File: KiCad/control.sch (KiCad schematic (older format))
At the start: 69 parts

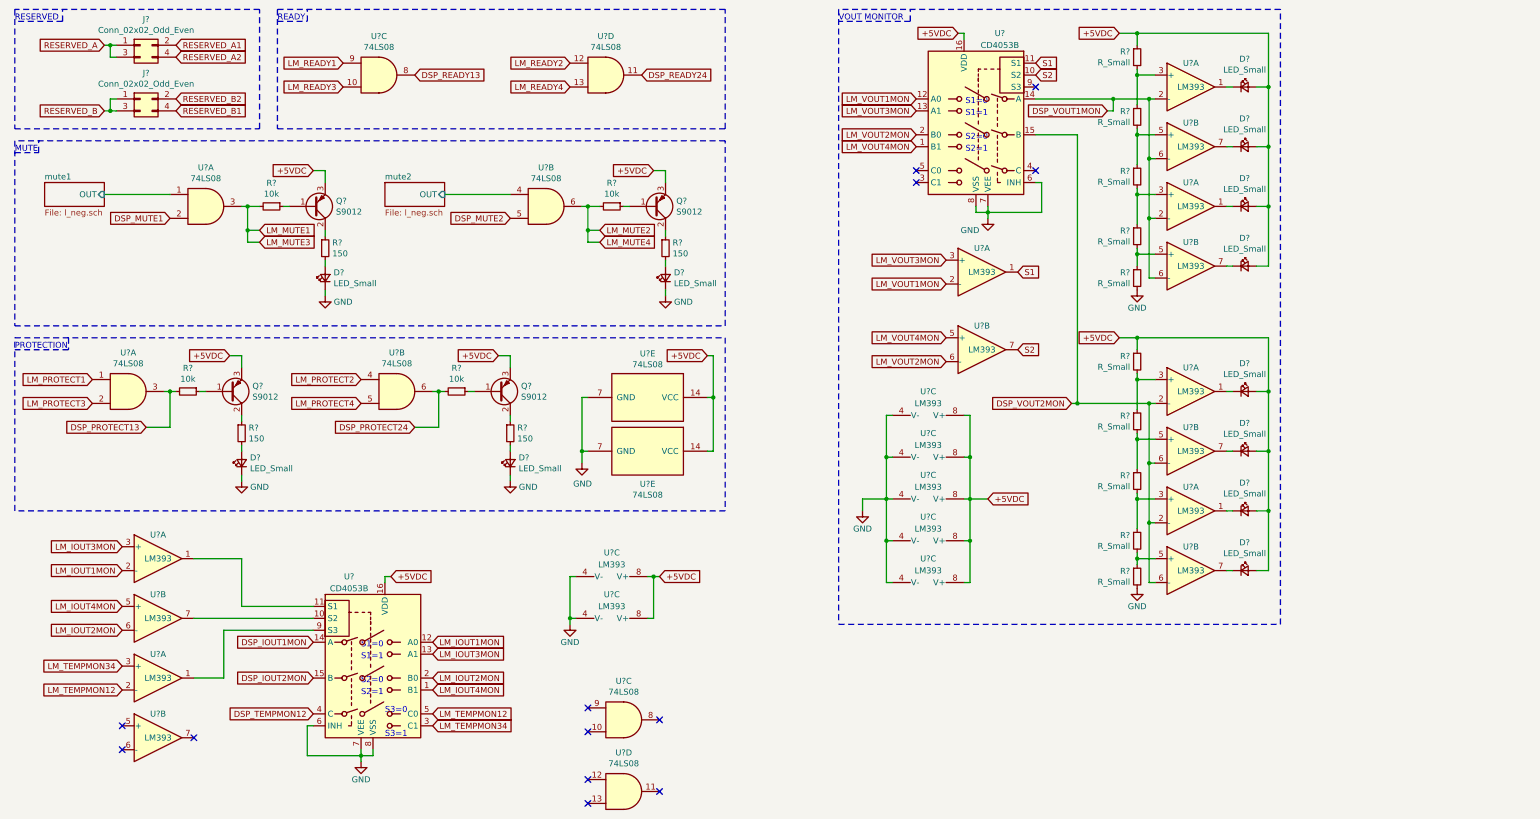
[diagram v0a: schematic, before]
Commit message: first commit
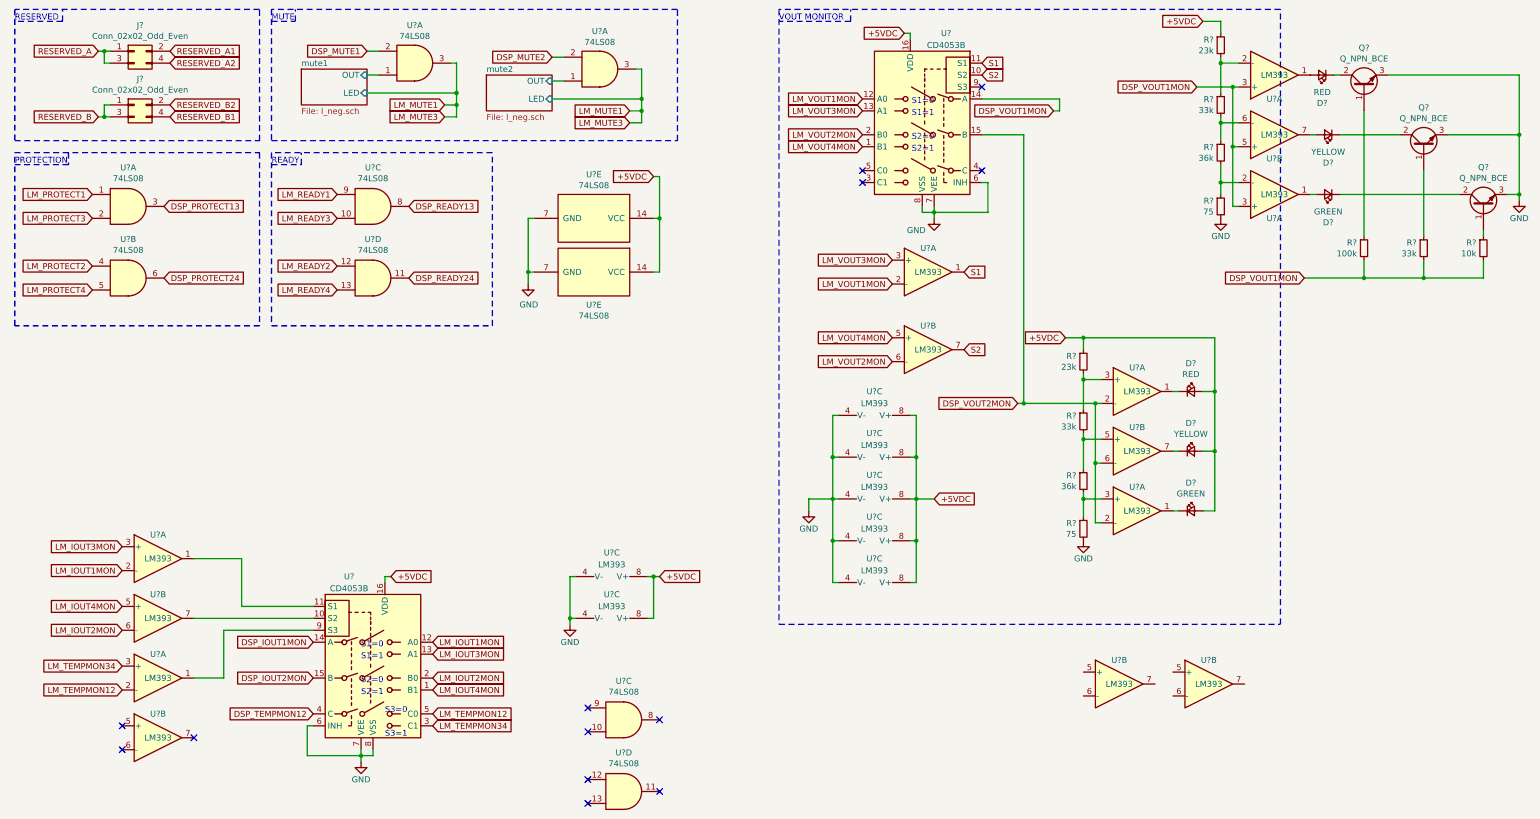
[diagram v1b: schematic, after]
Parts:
- removed D? (x6): LED_Small, symbol Device:LED_Small
- removed Q? (x4): S9012, symbol Device:Q_PNP_BCE
- removed R? (x4): 10k, symbol Device:R_Small
- removed R? (x4): 150, symbol Device:R_Small
- removed R? (x2): R_Small, symbol Device:R_Small
- removed U?: 74LS08, symbol 74xx:74LS08
- added Q? (x3): Q_NPN_BCE, symbol Device:Q_NPN_BCE
- added R?: 100k, symbol Device:R_Small
- added R?: 33k, symbol Device:R_Small
- added R?: 10k, symbol Device:R_Small
- added U?: 74LS08, symbol 74xx:74LS08
- D? (x2): value LED_Small -> RED
- D? (x2): value LED_Small -> YELLOW
- D? (x2): value LED_Small -> GREEN
- R? (x2): value R_Small -> 23k
- R? (x2): value R_Small -> 33k
- R? (x2): value R_Small -> 36k
- R? (x2): value R_Small -> 75
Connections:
- net +5VDC: no longer D?.2 (A), D?.2 (A), D?.2 (A)
- net DSP_MUTE2: now also U?.2
- net DSP_VOUT1MON: now also U?.3 (+), U?.3 (+), U?.5 (+), R?.2, R?.2, R?.2; no longer U?.2 (-), U?.2 (-), U?.6 (-), U?.6 (-)
- net DSP_VOUT2MON: no longer U?.6 (-)
- net GND: now also Q?.3 (E), Q?.3 (E), Q?.3 (E)
- net LM_MUTE1: now also U?.3
- net mute2/OUT: now also U?.1
- net at U?.5 (+): no longer R?.1 (x2)
- net at R?.2, U?.3 (+): now also R?.1
- net at U?.1: now also D?.2 (A); no longer D?.1 (K)
- net at R?.1, R?.2: now also U?.2 (-); no longer U?.3 (+)
- net at R?.1, R?.2: now also U?.6 (-); no longer U?.5 (+)
- net at U?.7: now also D?.2 (A); no longer D?.1 (K)
- net at R?.2: now also R?.1, U?.2 (-); no longer U?.3 (+)
- net at D?.1 (K): now also Q?.2 (C); no longer U?.1
- new net: D?.1 (K), Q?.2 (C) (x2)
- new net: D?.2 (A), U?.1
- new net: Q?.1 (B), R?.1 (x3)
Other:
- moved on the sheet: D?, J?, R?, U?, U?A, U?B, U?C, U?D, U?E
